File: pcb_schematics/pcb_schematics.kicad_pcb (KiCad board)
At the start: 2 copper layers, 140 x 108 mm, 56 parts, among them J1 CUE_SJ1-352XNG, J2 Conn_01x01_Pin, SW1 SW_Push, SW2 SW_Push, SW3 SW_Push, SW4 SW_Push, SW5 RotaryEncoder, SW6 RotaryEncoder, U1 RPi_Pico_TH, U2 RDA5807M_Module, U3 LM386, U4 LM386

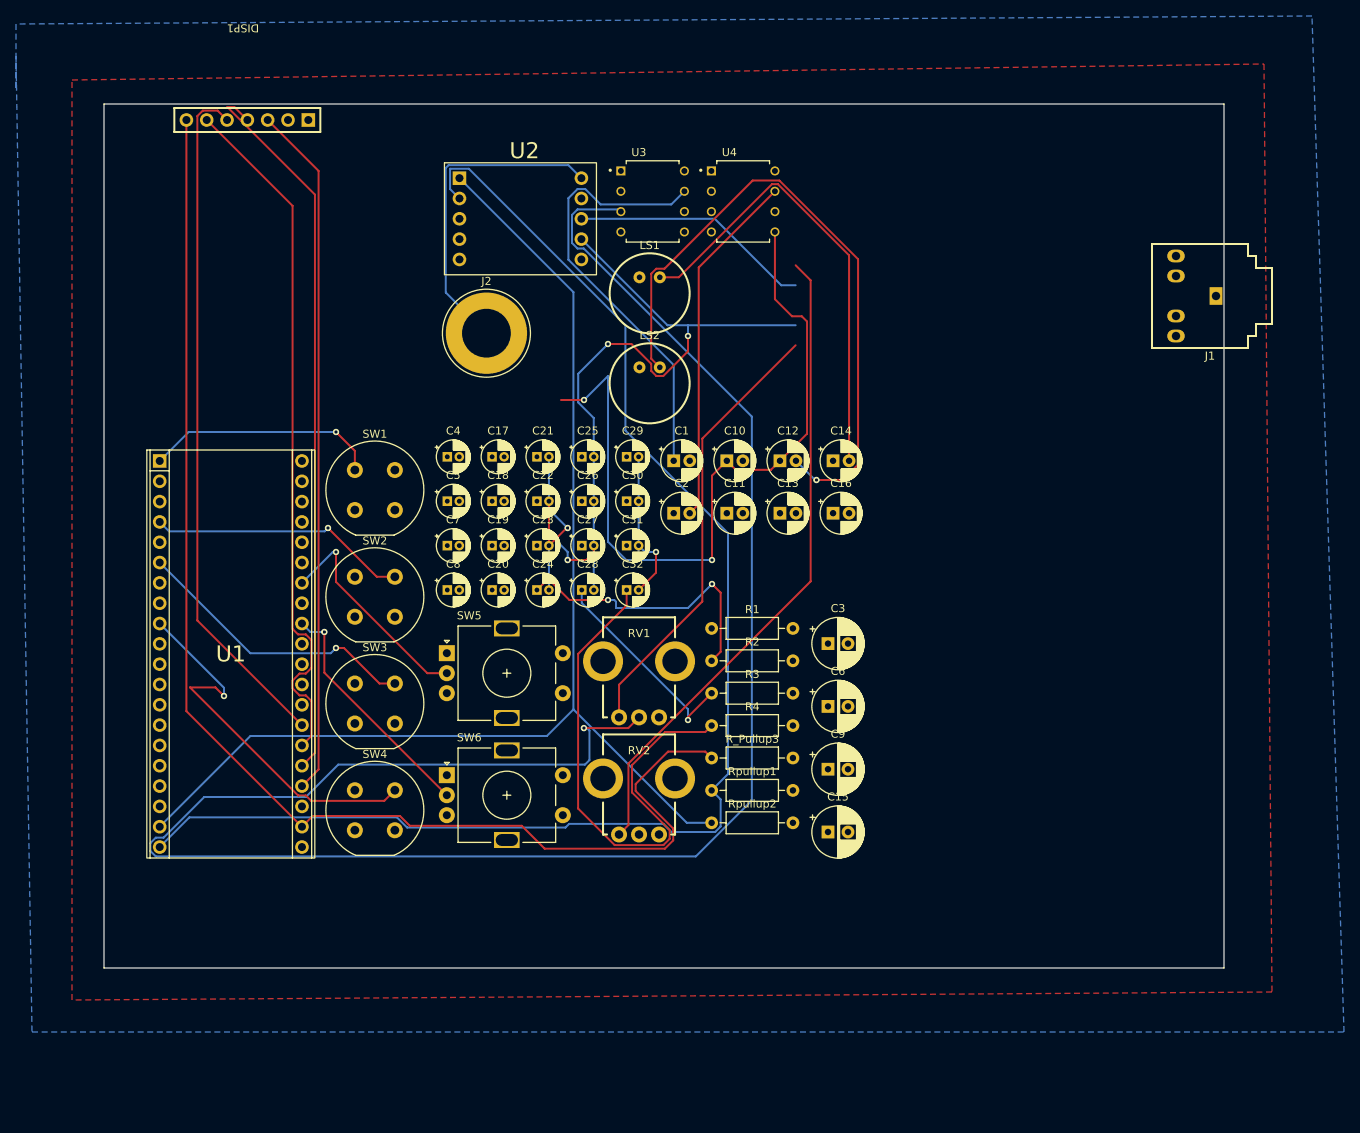
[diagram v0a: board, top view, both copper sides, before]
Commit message: Pcb (#1)
* Converted to connectors

* Updates PCb according to ROB's feedback

Added PCb layour according to the discussion with butoons and display on top and display below using front copper. Added Radio module using back copper. Speakers left to set up using back copper.

* compeltes PCB

Only the DRC has a couple errors

* Updates footprints in schematic

* Fixes errors in DRC

Adds SMD capacitors too

* Runs DRC and ERC again

* Accomodating usb cable

* Revision 3

Changed the amplifier and the rotary encoder schemtic. Needs work on pcb

* completes third version of PCB

* fixed issues mentioned by rob and brent

Fix iteration 1

* made changes based on changes requested

Fix iteration 2

* Submitted to JLCPCB

Modification with pcb_schematics being the final version.
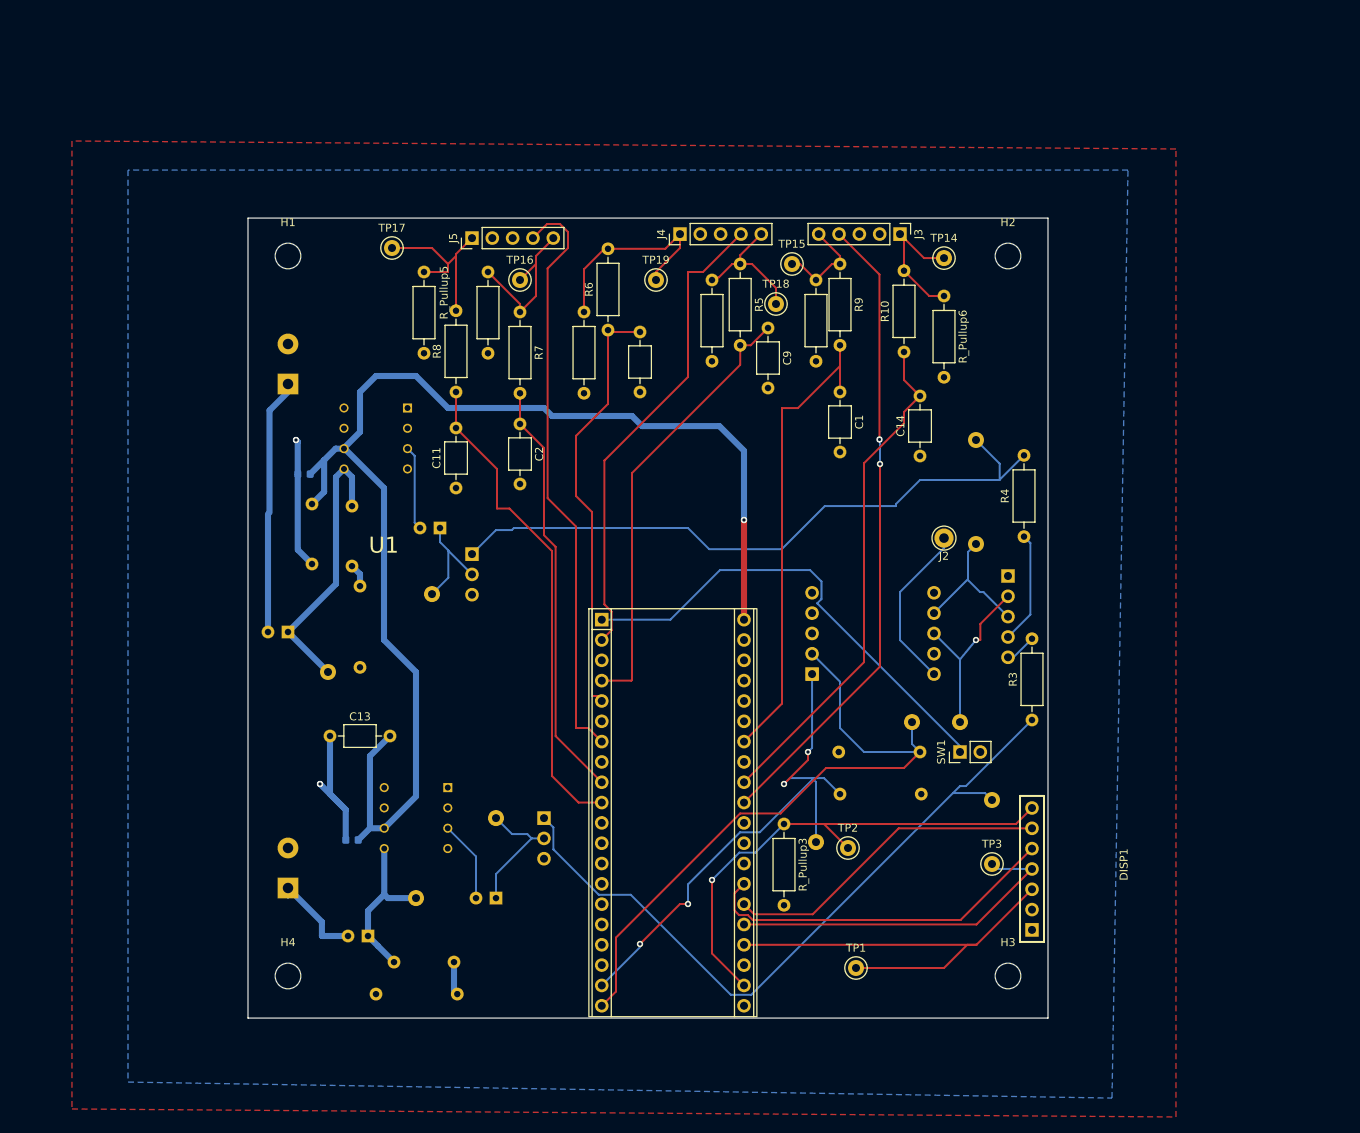
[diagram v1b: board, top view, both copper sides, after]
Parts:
- removed C17, C18, C19, C20, C21, C22, C23, C24, C25, C26, C27, C28, C29, C30, C31, C32: 10 nF, Capacitor_THT:CP_Radial_D4.0mm_P1.50mm
- removed SW2, SW3, SW4: SW_Push, Button_Switch_THT:Push_E-Switch_KS01Q01
- removed SW5, SW6: RotaryEncoder, Rotary_Encoder:RotaryEncoder_Alps_EC11E-Switch_Vertical_H20mm
- added H1: MountingHole, MountingHole:MountingHole_3.2mm_M3, F.Cu at (100.0, 48.0)
- added H2: MountingHole, MountingHole:MountingHole_3.2mm_M3, F.Cu at (190.0, 48.0)
- added H3: MountingHole, MountingHole:MountingHole_3.2mm_M3, F.Cu at (190.0, 138.0)
- added H4: MountingHole, MountingHole:MountingHole_3.2mm_M3, F.Cu at (100.0, 138.0)
- added J3: Conn_01x05, Connector_PinHeader_2.54mm:PinHeader_1x05_P2.54mm_Vertical, F.Cu at (176.5, 45.3)
- added J4: Conn_01x05, Connector_PinHeader_2.54mm:PinHeader_1x05_P2.54mm_Vertical, F.Cu at (149.0, 45.3)
- added J5: Conn_01x05, Connector_PinHeader_2.54mm:PinHeader_1x05_P2.54mm_Vertical, F.Cu at (123.0, 45.8)
- added R10: 10Ω, Resistor_THT:R_Axial_DIN0207_L6.3mm_D2.5mm_P10.16mm_Horizontal, F.Cu at (177.0, 60.0)
- added R5: 10Ω, Resistor_THT:R_Axial_DIN0207_L6.3mm_D2.5mm_P10.16mm_Horizontal, F.Cu at (156.5, 49.0)
- added R6: 10Ω, Resistor_THT:R_Axial_DIN0207_L6.3mm_D2.5mm_P10.16mm_Horizontal, F.Cu at (140.0, 57.3)
- added R7: 10kΩ, Resistor_THT:R_Axial_DIN0207_L6.3mm_D2.5mm_P10.16mm_Horizontal, F.Cu at (129.0, 55.0)
- added R8: 10kΩ, Resistor_THT:R_Axial_DIN0207_L6.3mm_D2.5mm_P10.16mm_Horizontal, F.Cu at (121.0, 65.0)
- added R9: 10Ω, Resistor_THT:R_Axial_DIN0207_L6.3mm_D2.5mm_P10.16mm_Horizontal, F.Cu at (169.0, 49.0)
- added R_Pullup1: 10kΩ, Resistor_THT:R_Axial_DIN0207_L6.3mm_D2.5mm_P10.16mm_Horizontal, F.Cu at (153.0, 51.0)
- added R_Pullup2: 10kΩ, Resistor_THT:R_Axial_DIN0207_L6.3mm_D2.5mm_P10.16mm_Horizontal, F.Cu at (137.0, 55.0)
- added R_Pullup4: 10kΩ, Resistor_THT:R_Axial_DIN0207_L6.3mm_D2.5mm_P10.16mm_Horizontal, F.Cu at (125.0, 50.0)
- added R_Pullup5: 10kΩ, Resistor_THT:R_Axial_DIN0207_L6.3mm_D2.5mm_P10.16mm_Horizontal, F.Cu at (117.0, 50.0)
- added R_Pullup6: 10kΩ, Resistor_THT:R_Axial_DIN0207_L6.3mm_D2.5mm_P10.16mm_Horizontal, F.Cu at (182.0, 53.0)
- added R_Pullup7: 10kΩ, Resistor_THT:R_Axial_DIN0207_L6.3mm_D2.5mm_P10.16mm_Horizontal, F.Cu at (166.0, 51.0)
- added TP1: TestPoint, TestPoint:TestPoint_Keystone_5000-5004_Miniature, F.Cu at (171.0, 137.0)
- added TP10: TestPoint, TestPoint:TestPoint_Keystone_5000-5004_Miniature, B.Cu at (184.0, 106.3)
- added TP11: TestPoint, TestPoint:TestPoint_Keystone_5000-5004_Miniature, B.Cu at (186.0, 84.0)
- added TP12: TestPoint, TestPoint:TestPoint_Keystone_5000-5004_Miniature, B.Cu at (186.0, 71.0)
- added TP13: TestPoint, TestPoint:TestPoint_Keystone_5000-5004_Miniature, B.Cu at (188.0, 116.0)
- added TP14: TestPoint, TestPoint:TestPoint_Keystone_5000-5004_Miniature, F.Cu at (182.0, 48.3)
- added TP15: TestPoint, TestPoint:TestPoint_Keystone_5000-5004_Miniature, F.Cu at (163.0, 49.0)
- added TP16: TestPoint, TestPoint:TestPoint_Keystone_5000-5004_Miniature, F.Cu at (129.0, 51.0)
- added TP17: TestPoint, TestPoint:TestPoint_Keystone_5000-5004_Miniature, F.Cu at (113.0, 47.0)
- added TP18: TestPoint, TestPoint:TestPoint_Keystone_5000-5004_Miniature, F.Cu at (161.0, 54.0)
- added TP19: TestPoint, TestPoint:TestPoint_Keystone_5000-5004_Miniature, F.Cu at (146.0, 51.0)
- added TP2: TestPoint, TestPoint:TestPoint_Keystone_5000-5004_Miniature, F.Cu at (170.0, 122.0)
- added TP3: TestPoint, TestPoint:TestPoint_Keystone_5000-5004_Miniature, F.Cu at (188.0, 124.0)
- added TP4: TestPoint, TestPoint:TestPoint_Keystone_5000-5004_Miniature, B.Cu at (166.0, 121.3)
- added TP5: TestPoint, TestPoint:TestPoint_Keystone_5000-5004_Miniature, B.Cu at (178.0, 106.3)
- added TP6: TestPoint, TestPoint:TestPoint_Keystone_5000-5004_Miniature, B.Cu at (118.0, 90.3)
- added TP7: TestPoint, TestPoint:TestPoint_Keystone_5000-5004_Miniature, B.Cu at (126.0, 118.3)
- added TP8: TestPoint, TestPoint:TestPoint_Keystone_5000-5004_Miniature, B.Cu at (116.0, 128.3)
- added TP9: TestPoint, TestPoint:TestPoint_Keystone_5000-5004_Miniature, B.Cu at (105.0, 100.0)
- C1, C10, C11, C14, C2: value 10 µF -> 0.01 µF; footprint Capacitor_THT:CP_Radial_D5.0mm_P2.00mm -> Capacitor_THT:C_Axial_L3.8mm_D2.6mm_P7.50mm_Horizontal
- C12: value 10 µF -> 0.1 µF; footprint Capacitor_THT:CP_Radial_D5.0mm_P2.00mm -> Capacitor_THT:C_Axial_L3.8mm_D2.6mm_P7.50mm_Horizontal; moved to B.Cu
- C13: value 10 µF -> 0.1 µF; footprint Capacitor_THT:CP_Radial_D5.0mm_P2.00mm -> Capacitor_THT:C_Axial_L3.8mm_D2.6mm_P7.50mm_Horizontal
- C15, C3, C6, R1, R2, Rpullup1, Rpullup2, U2, U3, U4: moved to B.Cu
- C16: value 10 µF -> 470 µF; footprint Capacitor_THT:CP_Radial_D5.0mm_P2.00mm -> Capacitor_THT:CP_Radial_D6.3mm_P2.50mm; moved to B.Cu
- C4, C5: value 10 nF -> 0.05 µF; footprint Capacitor_THT:CP_Radial_D4.0mm_P1.50mm -> Capacitor_THT:C_Axial_L3.8mm_D2.6mm_P7.50mm_Horizontal; moved to B.Cu
- C7, C8: value 10 nF -> 0.1 µF; footprint Capacitor_THT:CP_Radial_D4.0mm_P1.50mm -> Capacitor_SMD:C_0603_1608Metric; moved to B.Cu
- C9: value 470 µF -> 0.01 µF; footprint Capacitor_THT:CP_Radial_D6.3mm_P2.50mm -> Capacitor_THT:C_Axial_L3.8mm_D2.6mm_P7.50mm_Horizontal
- J1: footprint ECE:CUE_SJ1-352XNG -> Connector_PinHeader_2.54mm:PinHeader_1x05_P2.54mm_Vertical; moved to B.Cu
- J2: footprint Connector:Banana_Jack_1Pin -> Connector_Pin:Pin_D1.0mm_L10.0mm_LooseFit
- LS1, LS2: footprint ECE:CUE_CMA-4544PF-W -> TerminalBlock_Phoenix:TerminalBlock_Phoenix_MKDS-1,5-2_1x02_P5.00mm_Horizontal; moved to B.Cu
- R3, R4: value 10Ω -> 10 k
- RV1, RV2: footprint ECE:Bourns_PTV09_Horiz -> Connector_PinHeader_2.54mm:PinHeader_1x03_P2.54mm_Vertical; moved to B.Cu
- R_Pullup3: value 2kΩ -> 10kΩ
- SW1: footprint Button_Switch_THT:Push_E-Switch_KS01Q01 -> Connector_PinHeader_2.54mm:PinHeader_1x02_P2.54mm_Vertical
- moved DISP1 182.1 mm to (224.9, 142.4), turned to 90 degrees
- moved LS1 87.0 mm to (100.0, 127.0), turned to 90 degrees
- moved SW1 83.5 mm to (184.0, 110.0), turned to 90 degrees
- moved U3 82.6 mm to (116.0, 118.3), turned to 180 degrees
- moved U2 68.0 mm to (173.1, 95.2)
- moved C3 67.5 mm to (100.0, 95.0), turned to 180 degrees
- moved C6 64.3 mm to (110.0, 133.0), turned to 180 degrees
- moved C13 62.8 mm to (105.2, 108.0)
- moved J2 62.7 mm to (182.0, 83.3)
- moved C12 59.9 mm to (103.0, 86.5), turned to 90 degrees
- moved U1 58.7 mm to (148.1, 117.6)
- moved C5 58.0 mm to (113.2, 136.3)
- moved C9 55.7 mm to (160.0, 57.0), turned to -90 degrees
- moved U4 54.7 mm to (111.0, 70.8), turned to 180 degrees
- moved R2 52.4 mm to (121.2, 140.3), turned to 180 degrees
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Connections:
- C1 pad 1: Net-(U3-BYPASS) -> /ROT3A
- C10 pad 1: Net-(C10-Pad1) -> GND
- C10 pad 2: Net-(C10-Pad2) -> /ROT1A
- C11 pad 1: Net-(C10-Pad2) -> GND
- C11 pad 2: Net-(C11-Pad2) -> /ROT2B
- C12 pad 1: Net-(C10-Pad1) -> GND
- C12 pad 2: Net-(C11-Pad2) -> +5V
- C13 pad 1: Net-(C13-Pad1) -> GND
- C13 pad 2: Net-(C13-Pad2) -> +5V
- C14 pad 1: Net-(C13-Pad1) -> GND
- C14 pad 2: Net-(C14-Pad2) -> /ROT3B
- C15 pad 2: Net-(C14-Pad2) -> Net-(U3-+)
- C16 pad 1: Net-(C13-Pad2) -> Net-(C16-Pad1)
- C16 pad 2: Net-(C14-Pad2) -> Net-(U4-+)
- C2 pad 1: GND -> /ROT2A
- C2 pad 2: Net-(U4-BYPASS) -> GND
- C3 pad 1: Net-(C10-Pad1) -> Net-(C3-Pad1)
- C4 pad 1: Net-(C17-Pad1) -> Net-(C3-Pad1)
- C4 pad 2: Net-(C10-Pad1) -> Net-(C4-Pad2)
- C5 pad 1: Net-(C21-Pad1) -> Net-(C5-Pad1)
- C5 pad 2: Net-(C13-Pad1) -> Net-(C5-Pad2)
- C6 pad 1: Net-(C13-Pad1) -> Net-(C5-Pad1)
- C6 pad 2: Net-(C15-Pad1) -> Net-(C6-Pad2)
- C7 pad 1: Net-(C25-Pad1) -> GND
- C7 pad 2: /ROUT -> +5V
- C8 pad 1: Net-(C29-Pad1) -> GND
- C8 pad 2: /LOUT -> +5V
- C9 pad 1: Net-(C3-Pad2) -> /ROT1B
- C9 pad 2: Net-(C11-Pad2) -> GND
- J1 pad 2: /RSpeaker -> /LOUT
- J1 pad 3: /LSpeaker -> /ROUT
- J1 pad 4: /LOUT -> /RSpeaker
- J1 pad 5: /ROUT -> /LSpeaker
- LS1 pad 1: Net-(C14-Pad2) -> Net-(C6-Pad2)
- LS2 pad 1: Net-(C11-Pad2) -> Net-(C3-Pad2)
- R1 pad 1: Net-(C17-Pad1) -> Net-(C4-Pad2)
- R2 pad 1: Net-(C21-Pad1) -> Net-(C5-Pad2)
- R3 pad 1: Net-(C25-Pad1) -> Net-(R3-Pad1)
- R3 pad 2: GND -> /LSpeaker
- R4 pad 1: Net-(C29-Pad1) -> /RSpeaker
- R4 pad 2: GND -> Net-(R4-Pad2)
- RV1 pad 1: /LSpeaker -> Net-(R3-Pad1)
- RV1 pad 2: Net-(U3-+) -> Net-(C15-Pad1)
- RV2 pad 1: /RSpeaker -> Net-(R4-Pad2)
- RV2 pad 2: Net-(U4-+) -> Net-(C16-Pad1)
- U1 pad 10: unconnected-(U1-GP7-Pad10) -> /ROT2B
- U1 pad 2: unconnected-(U1-GP1-Pad2) -> /SW2
- U1 pad 31: unconnected-(U1-GP26/ADC0-Pad31) -> /SW3
- U1 pad 32: /RotB -> /ROT3B
- U1 pad 34: /RotA -> /ROT3A
- U1 pad 4: /SW2 -> /ROT1B
- U1 pad 5: unconnected-(U1-GP3-Pad5) -> /ROT1A
- U1 pad 6: /SW3 -> unconnected-(U1-GP4-Pad6)
- U1 pad 7: unconnected-(U1-GP5-Pad7) -> /SW4
- U1 pad 9: /SW4 -> /ROT2A
- U3 pad 5: Net-(C13-Pad1) -> Net-(C5-Pad1)
- U3 pad 6: /3V3 -> +5V
- U3 pad 7: Net-(U3-BYPASS) -> unconnected-(U3-BYPASS-Pad7)
- U4 pad 5: Net-(C10-Pad1) -> Net-(C3-Pad1)
- U4 pad 6: /3V3 -> +5V
- U4 pad 7: Net-(U4-BYPASS) -> unconnected-(U4-BYPASS-Pad7)
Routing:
- net Net-(U3-+): track 240.0 -> 10.2 mm, vias 1 -> 0
- net +5V: track 0.00 -> 162.8 mm, vias 0 -> 1
- net /CS: track 163.9 -> 63.1 mm, vias 0 -> 1
- net Net-(C10-Pad1): track 94.9 -> 0.00 mm, vias 2 -> 0
- net /I2CSCK: track 176.6 -> 83.6 mm
- net Net-(R3-Pad1): track 0.00 -> 91.7 mm
- net /I2CTX: track 153.2 -> 70.5 mm, vias 0 -> 4
- net Net-(R4-Pad2): track 0.00 -> 82.6 mm
- net Net-(C11-Pad2): track 82.1 -> 0.00 mm, vias 1 -> 0
- net /ROUT: track 89.0 -> 18.2 mm, vias 3 -> 0
- net /RSpeaker: track 81.8 -> 14.0 mm
- net Net-(C29-Pad1): track 66.7 -> 0.00 mm
- net /ROT3B: track 0.00 -> 63.7 mm
- net /ROT2B: track 0.00 -> 61.5 mm
- net /ROT3A: track 0.00 -> 58.9 mm
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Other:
- board size 140 x 108 mm -> 100 x 100 mm
- board text added: "Antenna"
- board text added: "Clock-Radio 29-06-25 Animish Murthy, Krishna Gupta 007, MI6"
